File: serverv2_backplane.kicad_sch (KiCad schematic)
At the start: 3 parts, among them U11 TPS65987DDJRSHR

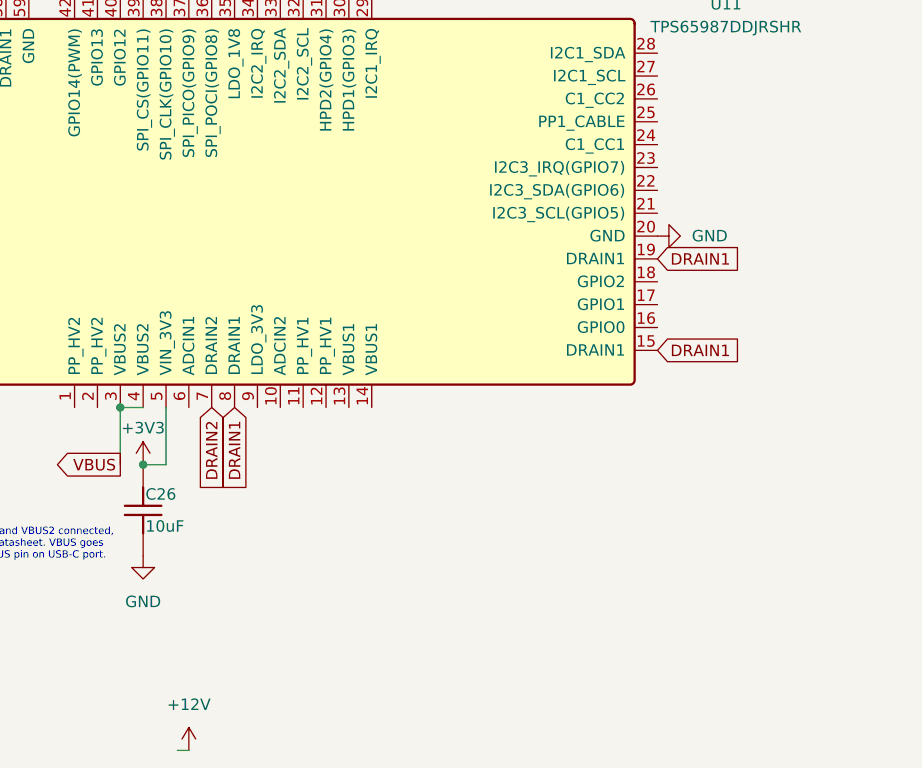
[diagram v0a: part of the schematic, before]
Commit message: Preliminary Revision of PS176 DP->HDMI Subsystem
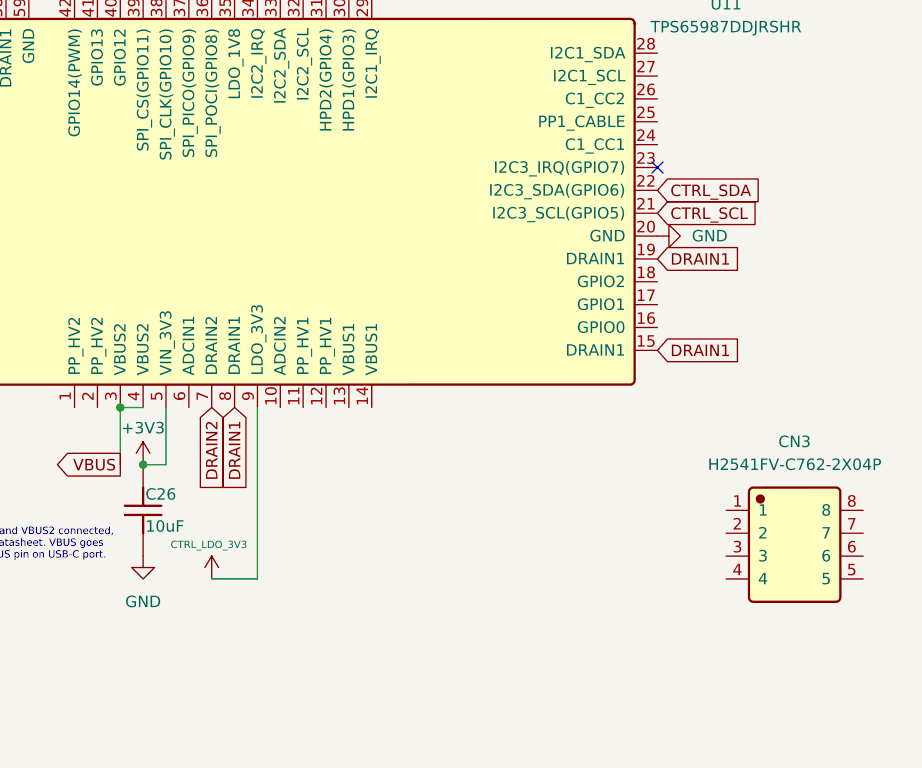
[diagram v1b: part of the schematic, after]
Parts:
- added CN3: H2541FV-C762-2X04P, JLCImport:H2541FV-C762-2X04P, symbol JLCImport:H2541FV-C762-2X04P
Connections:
- net CTRL_SCL: now reaches U11.21 (I2C3_SCL(GPIO5))
- net CTRL_SDA: now reaches U11.22 (I2C3_SDA(GPIO6))
- net CTRL_LDO_3V3: now reaches U11.9 (LDO_3V3)
- no-connect marks 2 -> 3
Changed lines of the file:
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@@
+	)
+	(no_connect
+		(at 201.93 48.26)
 	)
 	(no_connect
@@
 	(wire
 		(pts
+			(xy 157.48 93.98) (xy 157.48 74.93)
+		)
+		(stroke
+			(width 0)
+			(type default)
+		)
+	)
+	(wire
+		(pts
+			(xy 152.4 93.98) (xy 157.48 93.98)
+		)
+		(stroke
+			(width 0)
+			(type default)
+		)
+	)
+	(wire
+		(pts
 			(xy 41.91 26.67) (xy 44.45 26.67)
 		)
@@
 		(pts
 			(xy 59.69 26.67) (xy 59.69 34.29)
-		)
-		(stroke
-			(width 0)
-			(type default)
-		)
-	)
-	(wire
-		(pts
-			(xy 149.86 113.03) (xy 148.59 113.03)
 		)
 		(stroke
@@
 		)
 	)
+	(global_label "CTRL_SDA"
+		(shape input)
+		(at 201.93 50.8 0)
+		(fields_autoplaced yes)
+		(effects
+			(font
+				(size 1.27 1.27)
+			)
+			(justify left)
+		)
+		(property "Intersheetrefs" "${INTERSHEET_REFS}"
+			(at 213.9866 50.8 0)
+			(hide yes)
+			(show_name no)
+			(do_not_autoplace no)
+			(effects
+				(font
+					(size 1.27 1.27)
+				)
+				(justify left)
+			)
+		)
+	)
 	(global_label "DRAIN1"
 		(shape input)
@@
 				)
 				(justify right)
+			)
+		)
+	)
+	(global_label "CTRL_SCL"
+		(shape input)
+		(at 201.93 53.34 0)
+		(fields_autoplaced yes)
+		(effects
+			(font
+				(size 1.27 1.27)
+			)
+			(justify left)
+		)
+		(property "Intersheetrefs" "${INTERSHEET_REFS}"
+			(at 213.9261 53.34 0)
+			(hide yes)
+			(show_name no)
+			(do_not_autoplace no)
+			(effects
+				(font
+					(size 1.27 1.27)
+				)
+				(justify left)
 			)
 		)
@@
 	)
 	(symbol
+		(lib_id "power:+3V3")
+		(at 152.4 93.98 0)
+		(unit 1)
+		(body_style 1)
+		(exclude_from_sim no)
+		(in_bom yes)
+		(on_board yes)
+		(in_pos_files yes)
+		(dnp no)
+		(property "Reference" "#PWR0164"
+			(at 152.4 97.79 0)
+			(hide yes)
+			(show_name no)
+			(do_not_autoplace no)
+			(effects
+				(font
+					(size 1.27 1.27)
+				)
+			)
+		)
+		(property "Value" "CTRL_LDO_3V3"
+			(at 147.828 90.17 0)
+			(show_name no)
+			(do_not_autoplace no)
+			(effects
+				(font
+					(size 0.8128 0.8128)
+				)
+				(justify left)
+			)
+		)
+		(property "Footprint" ""
+			(at 152.4 93.98 0)
+			(hide yes)
+			(show_name no)
+			(do_not_autoplace no)
+			(effects
+				(font
+					(size 1.27 1.27)
+				)
+			)
+		)
+		(property "Datasheet" ""
+			(at 152.4 93.98 0)
+			(hide yes)
+			(show_name no)
+			(do_not_autoplace no)
+			(effects
+				(font
+					(size 1.27 1.27)
+				)
+			)
+		)
+		(property "Description" "Power symbol creates a global label with name \"+3V3\""
+			(at 152.4 93.98 0)
+			(hide yes)
+			(show_name no)
+			(do_not_autoplace no)
+			(effects
+				(font
+					(size 1.27 1.27)
+				)
+			)
+		)
+		(pin "1"
+		)
+		(instances
+			(project "serverv2_backplane"
+				(path "/d38d6818-cf53-410d-afa3-a75a85b7c05a"
+					(reference "#PWR0164")
+					(unit 1)
+				)
+			)
+		)
+	)
+	(symbol
 		(lib_id "power:GND")
 		(at 134.62 22.86 0)
@@
 	)
 	(symbol
-		(lib_id "power:+5V")
-		(at 149.86 113.03 0)
+		(lib_id "JLCImport:H2541FV-C762-2X04P")
+		(at 217.17 90.17 0)
 		(unit 1)
 		(body_style 1)
@@
 		(dnp no)
 		(fields_autoplaced yes)
-		(property "Reference" "#PWR0144"
-			(at 149.86 116.84 0)
-			(hide yes)
-			(show_name no)
-			(do_not_autoplace no)
-			(effects
-				(font
-					(size 1.27 1.27)
-				)
-			)
-		)
-		(property "Value" "+12V"
-			(at 149.86 107.95 0)
-			(show_name no)
-			(do_not_autoplace no)
-			(effects
-				(font
-					(size 1.27 1.27)
-				)
-			)
-		)
-		(property "Footprint" ""
-			(at 149.86 113.03 0)
-			(hide yes)
-			(show_name no)
-			(do_not_autoplace no)
-			(effects
-				(font
-					(size 1.27 1.27)
-				)
-			)
-		)
-		(property "Datasheet" ""
-			(at 149.86 113.03 0)
-			(hide yes)
-			(show_name no)
-			(do_not_autoplace no)
-			(effects
-				(font
-					(size 1.27 1.27)
-				)
-			)
-		)
-		(property "Description" "Power symbol creates a global label with name \"+5V\""
-			(at 149.86 113.03 0)
-			(hide yes)
-			(show_name no)
-			(do_not_autoplace no)
-			(effects
-				(font
-					(size 1.27 1.27)
-				)
-			)
+		(property "Reference" "CN3"
+			(at 217.17 78.74 0)
+			(show_name no)
+			(do_not_autoplace no)
+			(effects
+				(font
+					(size 1.27 1.27)
+				)
+			)
+		)
+		(property "Value" "H2541FV-C762-2X04P"
+			(at 217.17 81.28 0)
+			(show_name no)
+			(do_not_autoplace no)
+			(effects
+				(font
+					(size 1.27 1.27)
+				)
+			)
+		)
+		(property "Footprint" "JLCImport:H2541FV-C762-2X04P"
+			(at 217.17 90.17 0)
+			(hide yes)
+			(show_name no)
+			(do_not_autoplace no)
+			(effects
+				(font
+					(size 1.27 1.27)
+				)
+			)
+		)
+		(property "Datasheet" "https://www.lcsc.com/datasheet/lcsc_datasheet_2405141422_HanElectricity-H2541FV-C762-2x04P_C22387106.pdf"
+			(at 217.17 90.17 0)
+			(hide yes)
+			(show_name no)
+			(do_not_autoplace no)
+			(effects
+				(font
+					(size 1.27 1.27)
+				)
+			)
+		)
+		(property "Description" "-55℃~+105℃ 2.54mm 7.62mm 8P DIP Phosphor bronze Square Hole DIP-8 IC / Transistor Socket ROHS"
+			(at 217.17 90.17 0)
+			(hide yes)
+			(show_name no)
+			(do_not_autoplace no)
+			(effects
+				(font
+					(size 1.27 1.27)
+				)
+			)
+		)
+		(property "LCSC" "C22387106"
+			(at 217.17 90.17 0)
+			(hide yes)
+			(show_name no)
+			(do_not_autoplace no)
+			(effects
+				(font
+					(size 1.27 1.27)
+				)
+			)
+		)
+		(property "Manufacturer" "HanElectricity"
+			(at 217.17 90.17 0)
+			(hide yes)
+			(show_name no)
+			(do_not_autoplace no)
+			(effects
+				(font
+					(size 1.27 1.27)
+				)
+			)
+		)
+		(property "Manufacturer Part" "H2541FV-C762-2x04P"
+			(at 217.17 90.17 0)
+			(hide yes)
+			(show_name no)
+			(do_not_autoplace no)
+			(effects
+				(font
+					(size 1.27 1.27)
+				)
+			)
+		)
+		(pin "2"
 		)
 		(pin "1"
+		)
+		(pin "8"
+		)
+		(pin "3"
+		)
+		(pin "5"
+		)
+		(pin "7"
+		)
+		(pin "4"
+		)
+		(pin "6"
 		)
 		(instances
 			(project "serverv2_backplane"
 				(path "/d38d6818-cf53-410d-afa3-a75a85b7c05a"
-					(reference "#PWR0144")
+					(reference "CN3")
 					(unit 1)
 				)
